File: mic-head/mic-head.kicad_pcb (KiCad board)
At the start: 2 copper layers, 22 x 40 mm, 16 parts, among them J1 Loetpads_Kabel_5x, U1 TPS7A2028, U2 OPA2325

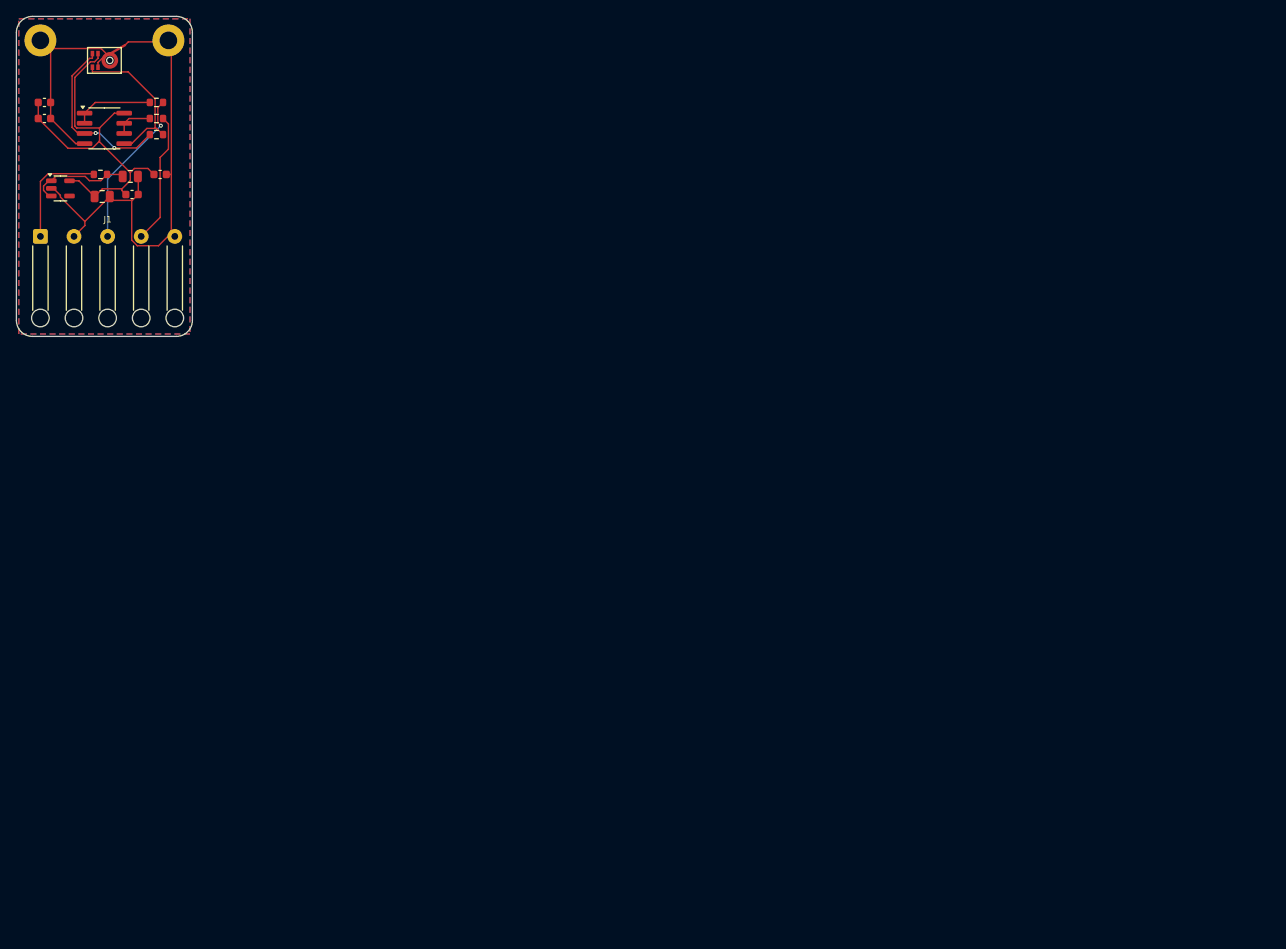
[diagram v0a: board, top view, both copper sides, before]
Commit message: modified:   01-power.kicad_sch 	modified:   02-analog.kicad_sch 	modified:   03-adc.kicad_sch 	modified:   04-mcu.kicad_sch 	modified:   05-io.kicad_sch 	modified:   exhaust-mic.kicad_pcb 	modified:   exhaust-mic.kicad_pro 	modified:   exhaust-mic.kicad_sch 	modified:   mic-head/mic-head.kicad_pcb 	modified:   mic-head/mic-head.kicad_pro 	modified:   mic-head/mic-head.kicad_sch 	new file:   ~exhaust-mic.kicad_pro.lck
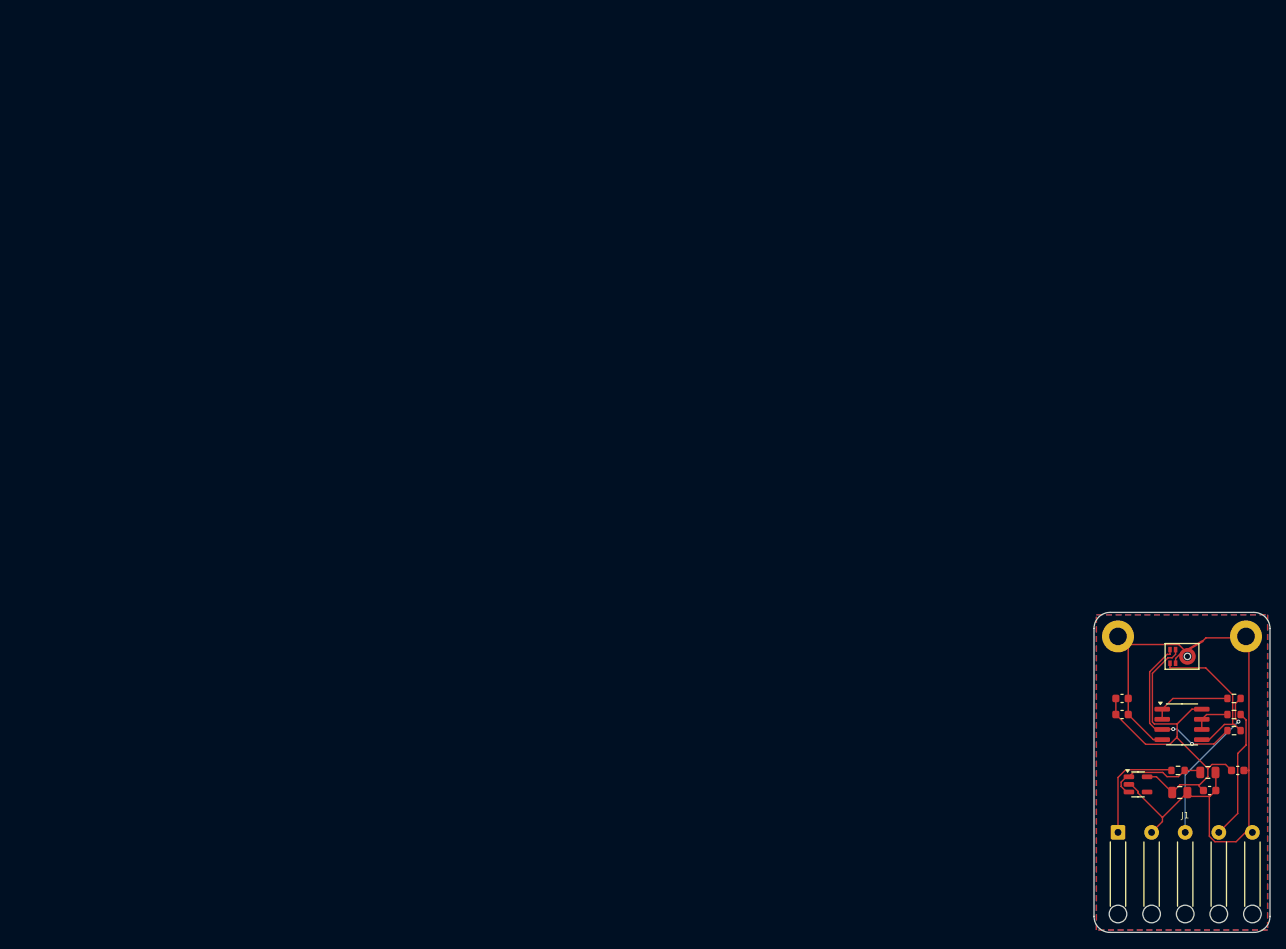
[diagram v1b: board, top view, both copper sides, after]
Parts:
- moved C4 153.9 mm to (145.4, 97.0)
- moved C5 153.9 mm to (138.2, 85.3)
- moved C6 153.9 mm to (138.2, 87.3)
- moved R1 153.9 mm to (152.2, 85.3)
- moved R2 153.9 mm to (152.2, 87.3)
- moved R3 153.9 mm to (152.2, 89.3)
- moved C1 153.9 mm to (148.9, 94.5)
- moved C3 153.9 mm to (152.7, 94.3)
- moved C7 153.9 mm to (149.2, 96.8)
- moved FB1 153.9 mm to (145.2, 94.3)
- moved H1 153.9 mm to (137.7, 77.5)
- moved H2 153.9 mm to (153.7, 77.5)
- moved J1 153.9 mm to (137.7, 102.0)
- moved MK1 153.9 mm to (145.7, 80.0)
- moved U1 153.9 mm to (140.2, 96.0)
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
